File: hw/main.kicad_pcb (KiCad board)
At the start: 2 copper layers, 110 x 85 mm, 106 parts, among them J1 UART_01X03, J2 SWD_01X04, J3 SWD_01X04, J4 IDC_02X07, J5 IDC_02X07, J6 IDC_02X03, J7 IDC_02X13, J8 SMA, J9 IDC_02X05, SW1 LCD_BTN, U1 STM32F405RGTx, U10 MCP1826S, U11 OSRB38C9BA, U12 74AHC1G08, U13 74AHC1G08, U2 LM4861, U3 AD8542, U4 LM4861, U5 AD8542, U6 STM32F405RGTx, U7 HM-TRP-869S, U8 ULN2003, U9 MCP1826S

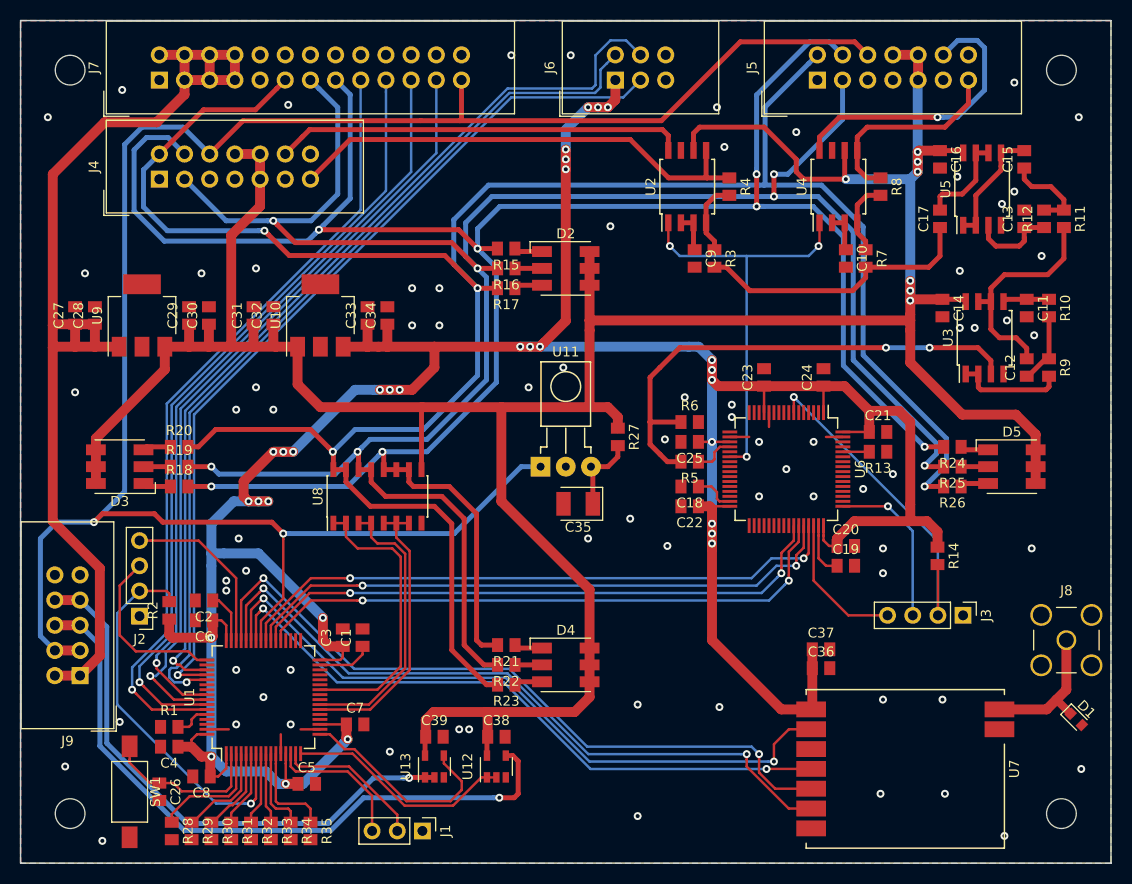
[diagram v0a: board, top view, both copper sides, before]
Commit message: updated pcb
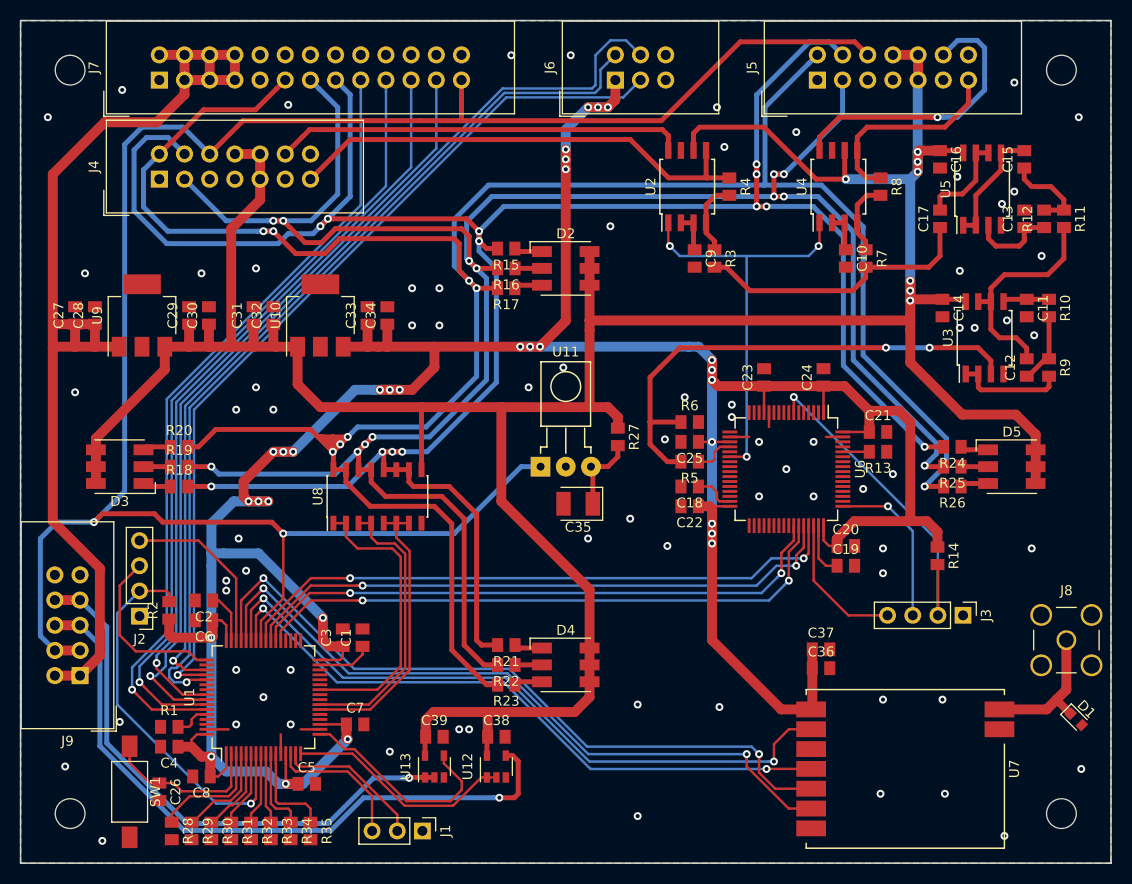
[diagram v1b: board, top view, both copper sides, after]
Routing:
- net /Back/LED_PWM_R: track 239.6 -> 254.1 mm, vias 4 -> 8
- net /Back/LED_PWM_B: track 238.3 -> 246.7 mm, vias 7 -> 13
- net /Back/LED_PWM_G: track 225.5 -> 232.0 mm, vias 7 -> 13
- net +5V: track 312.7 -> 311.9 mm
